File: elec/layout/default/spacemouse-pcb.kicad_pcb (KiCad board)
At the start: 2 copper layers, 78 x 78 mm, 11 parts

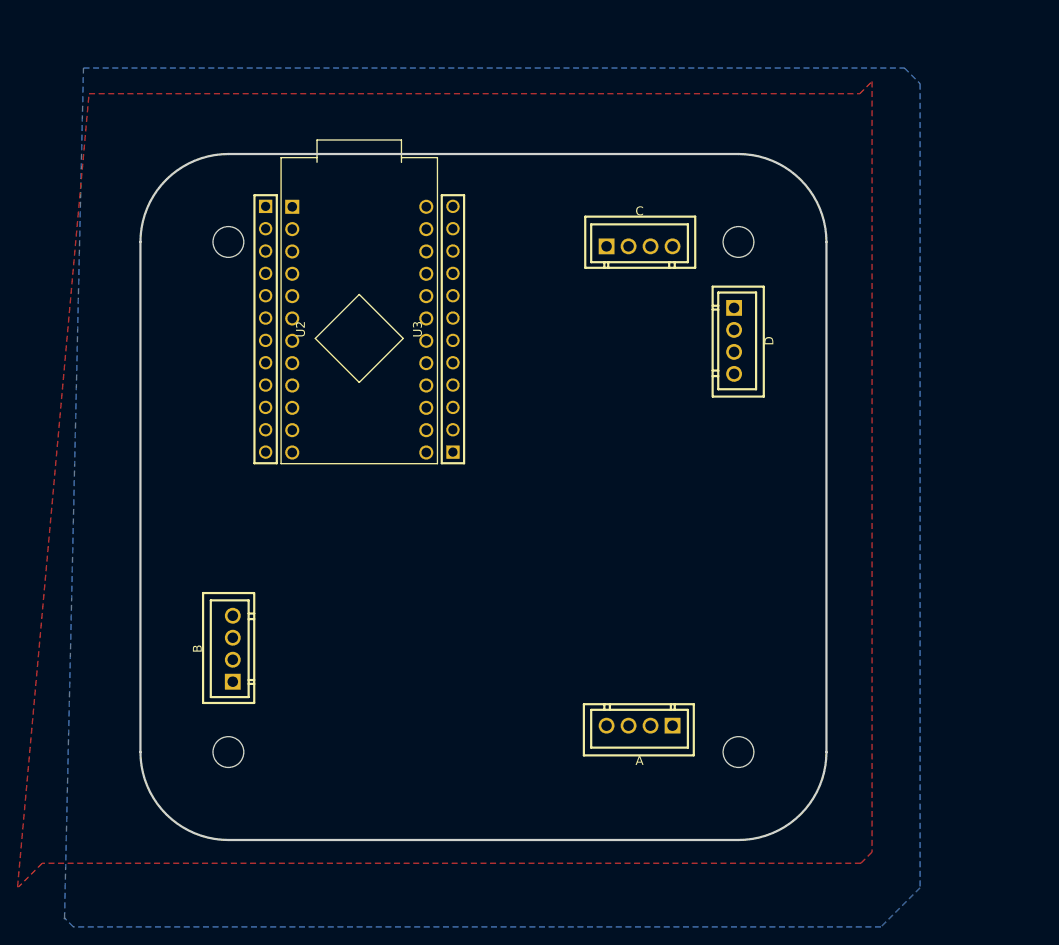
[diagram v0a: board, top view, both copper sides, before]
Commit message: basic complete
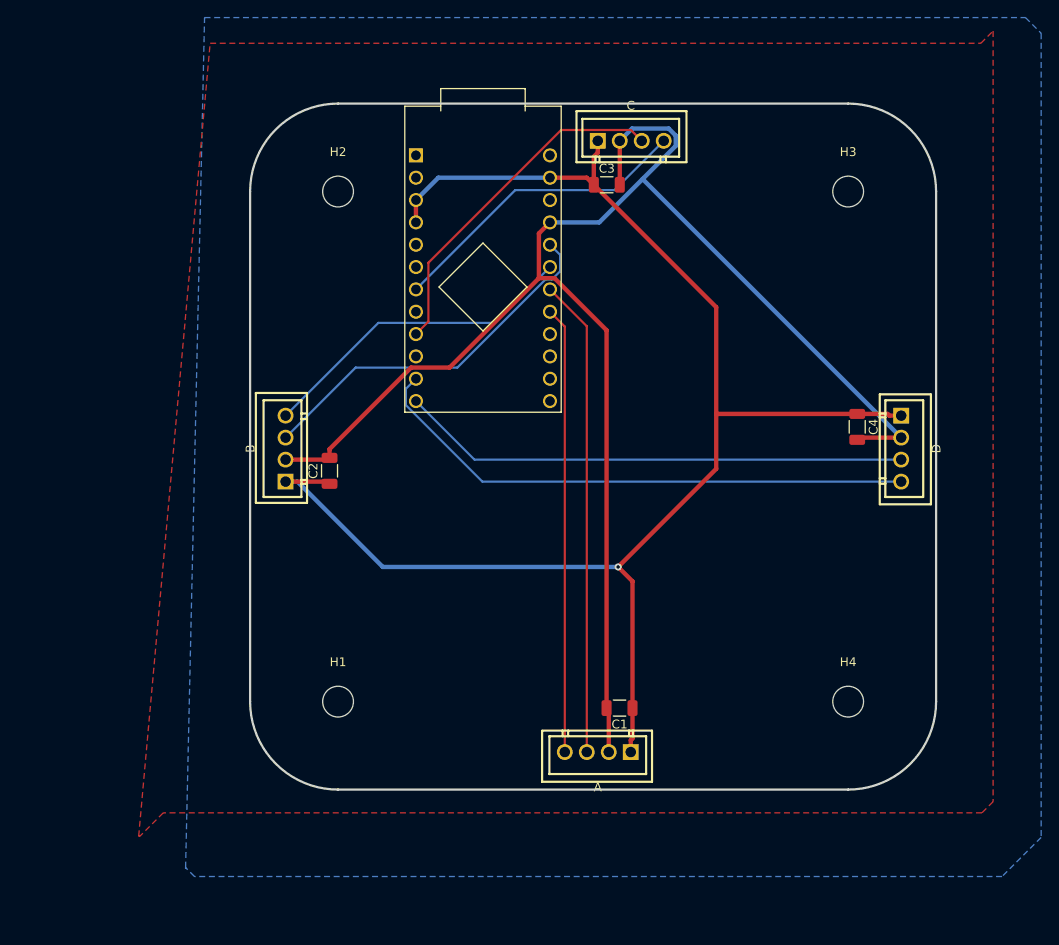
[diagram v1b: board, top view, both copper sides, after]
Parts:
- removed ? (x4): , 
- removed U2, U3: , lib:HDR-TH_12P-P2.54-V-M
- added C1: 50V 100nF X7R ±10% 1206 Multilayer Ceramic Capacitors MLCC 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, lib:C1206, F.Cu at (152.5, 129.5)
- added C2: 50V 100nF X7R ±10% 1206 Multilayer Ceramic Capacitors MLCC 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, lib:C1206, F.Cu at (119.5, 102.5)
- added C3: 50V 100nF X7R ±10% 1206 Multilayer Ceramic Capacitors MLCC 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, lib:C1206, F.Cu at (151.0, 70.0)
- added C4: 50V 100nF X7R ±10% 1206 Multilayer Ceramic Capacitors MLCC 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, lib:C1206, F.Cu at (179.5, 97.5)
- added H1: MountingHole_3.5mm, MountingHole:MountingHole_3.5mm, F.Cu at (120.5, 128.8)
- added H2: MountingHole_3.5mm, MountingHole:MountingHole_3.5mm, F.Cu at (120.5, 70.8)
- added H3: MountingHole_3.5mm, MountingHole:MountingHole_3.5mm, F.Cu at (178.5, 70.8)
- added H4: MountingHole_3.5mm, MountingHole:MountingHole_3.5mm, F.Cu at (178.5, 128.8)
- moved B 23.5 mm to (114.5, 100.0)
- moved D 22.6 mm to (184.5, 100.0)
- moved U1 15.2 mm to (136.9, 80.6)
- moved C 12.0 mm to (153.8, 65.0)
- moved A 5.62 mm to (150.0, 134.5)
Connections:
- A pad 3: joyA-_3 -> a1
- A pad 4: joyA-_4 -> a0
- B pad 3: joyB-_3 -> a3
- B pad 4: joyB-_4 -> a2
- C pad 3: joyC-_3 -> a7
- C pad 4: joyC-_4 -> a6
- D pad 3: joyD-_3 -> a9
- D pad 4: joyD-_4 -> a8
- U1 pad 11: (no net) -> a8
- U1 pad 12: (no net) -> a9
- U1 pad 17: (no net) -> a0
- U1 pad 18: (no net) -> a1
- U1 pad 19: (no net) -> a2
- U1 pad 20: (no net) -> a3
- U1 pad 7: (no net) -> a6
- U1 pad 9: (no net) -> a7
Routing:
- net vcc: track 0.00 -> 181.1 mm
- net gnd: track 0.00 -> 173.0 mm, vias 0 -> 1
- net a8: track 0.00 -> 63.4 mm
- net a9: track 0.00 -> 57.9 mm
- net a1: track 0.00 -> 54.3 mm
- net a0: track 0.00 -> 50.8 mm
- net a3: track 0.00 -> 42.6 mm
- net a7: track 0.00 -> 39.7 mm
- net a2: track 0.00 -> 37.1 mm
- net a6: track 0.00 -> 35.2 mm
